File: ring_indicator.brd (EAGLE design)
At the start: 53 x 36.8 mm, 19 parts, among them Q2 BUZ11

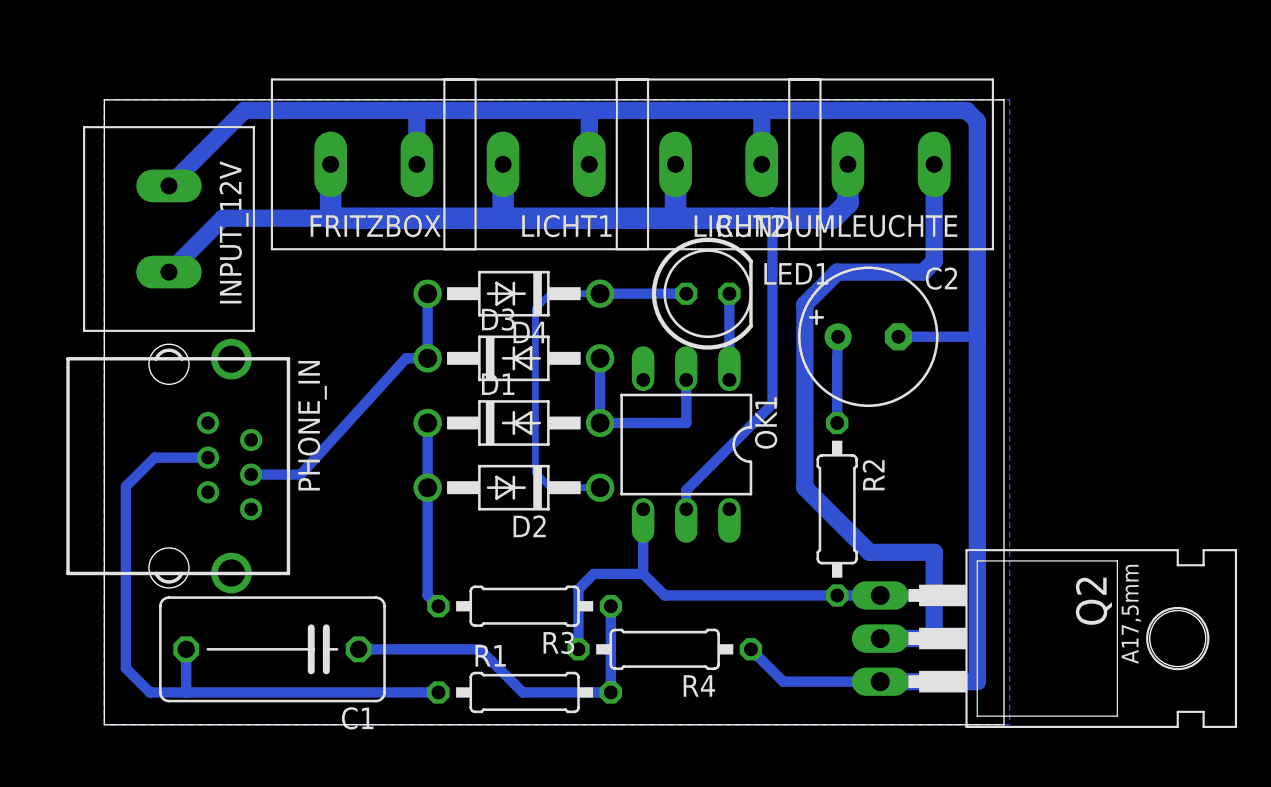
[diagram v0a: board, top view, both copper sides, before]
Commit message: v0.2.2-layout simplified
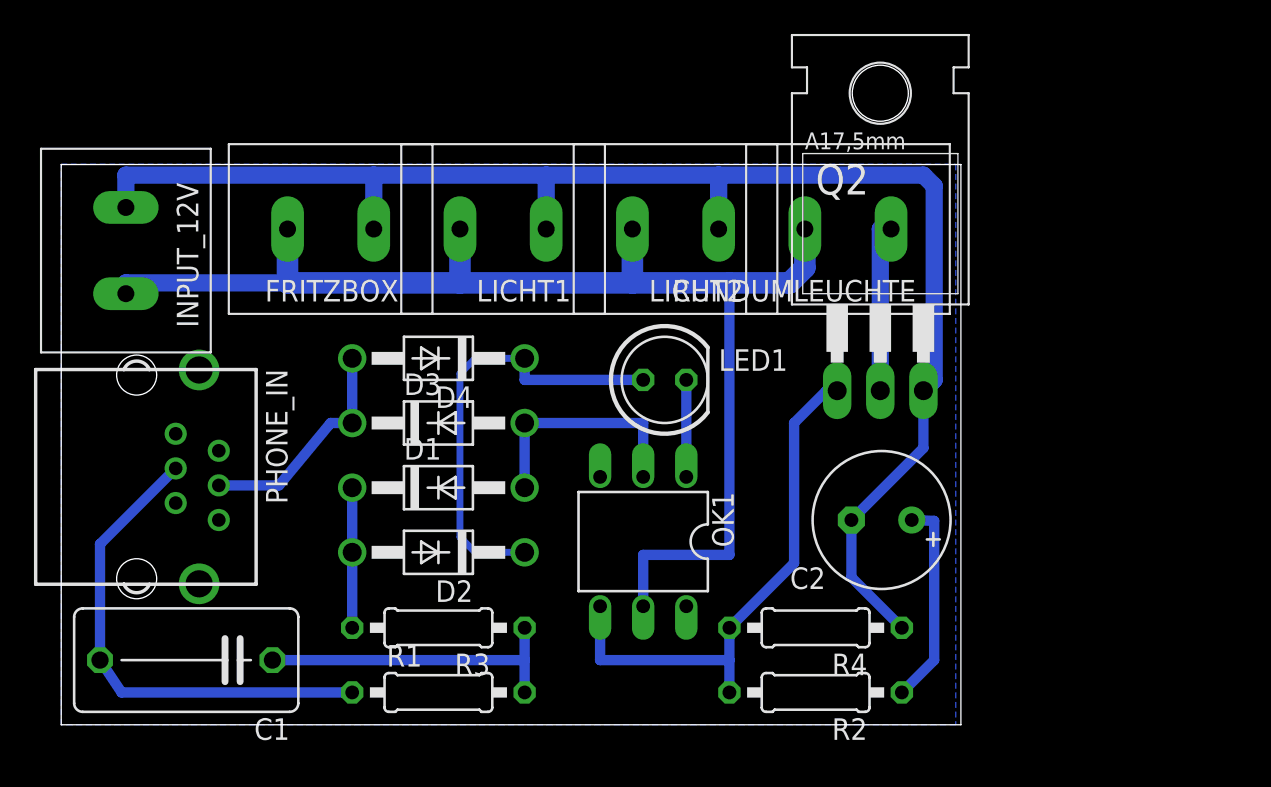
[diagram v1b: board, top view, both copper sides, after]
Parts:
- R4: value 100k -> 50k
- moved Q2 21.9 mm to (48.3, 26.0), turned to 0 degrees
- moved R2 10.9 mm to (44.5, 1.91), turned to 180 degrees
- moved C2 10.8 mm to (48.3, 12.1), turned to 180 degrees
- moved R4 8.98 mm to (44.5, 5.71)
- moved OK1 6.25 mm to (34.3, 10.8)
- moved D1 5.85 mm to (22.2, 14.0)
- moved D2 5.85 mm to (22.2, 10.2)
- moved D3 5.85 mm to (22.2, 17.8)
- moved D4 5.85 mm to (22.2, 21.6)
- moved LED1 5.68 mm to (35.6, 20.3)
- moved R3 5.24 mm to (22.2, 5.71)
- moved C1 5.12 mm to (7.37, 3.81)
- moved R1 5.08 mm to (22.2, 1.91)
- moved RUNDUMLEUCHTE 4.58 mm to (46.4, 29.2)
- moved FRITZBOX 4.58 mm to (15.9, 29.2)
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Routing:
- net N$6: track 42.6 -> 10.2 mm
- net GND: track 111.0 -> 88.6 mm
- net A: track 37.8 -> 29.0 mm
- net N$10: track 5.08 -> 12.2 mm
- net N$9: track 26.0 -> 31.6 mm
- net VCC: track 72.7 -> 76.9 mm
- net B: track 17.2 -> 13.4 mm
- net N$4: track 23.1 -> 26.3 mm
- net N$3: track 11.1 -> 8.26 mm
- net N$5: track 11.4 -> 14.0 mm
- net N$1: track 21.0 -> 18.7 mm
- net N$2: track 5.08 -> 5.71 mm
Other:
- board size 53 x 36.8 mm -> 53 x 33 mm
